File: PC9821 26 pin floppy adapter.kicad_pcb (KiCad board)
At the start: 2 copper layers, 52.7 x 28.6 mm, 3 parts

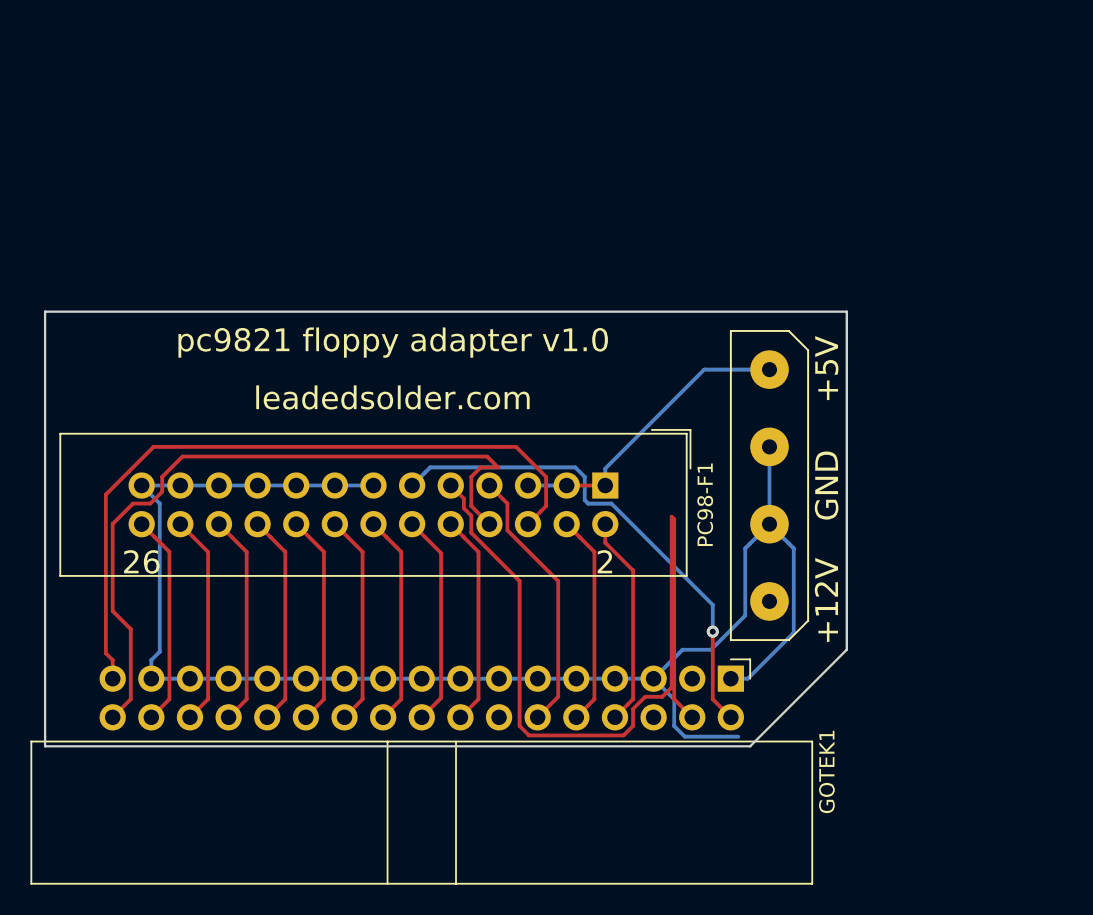
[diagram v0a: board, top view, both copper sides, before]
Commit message: Final version that I just sent off to Osh
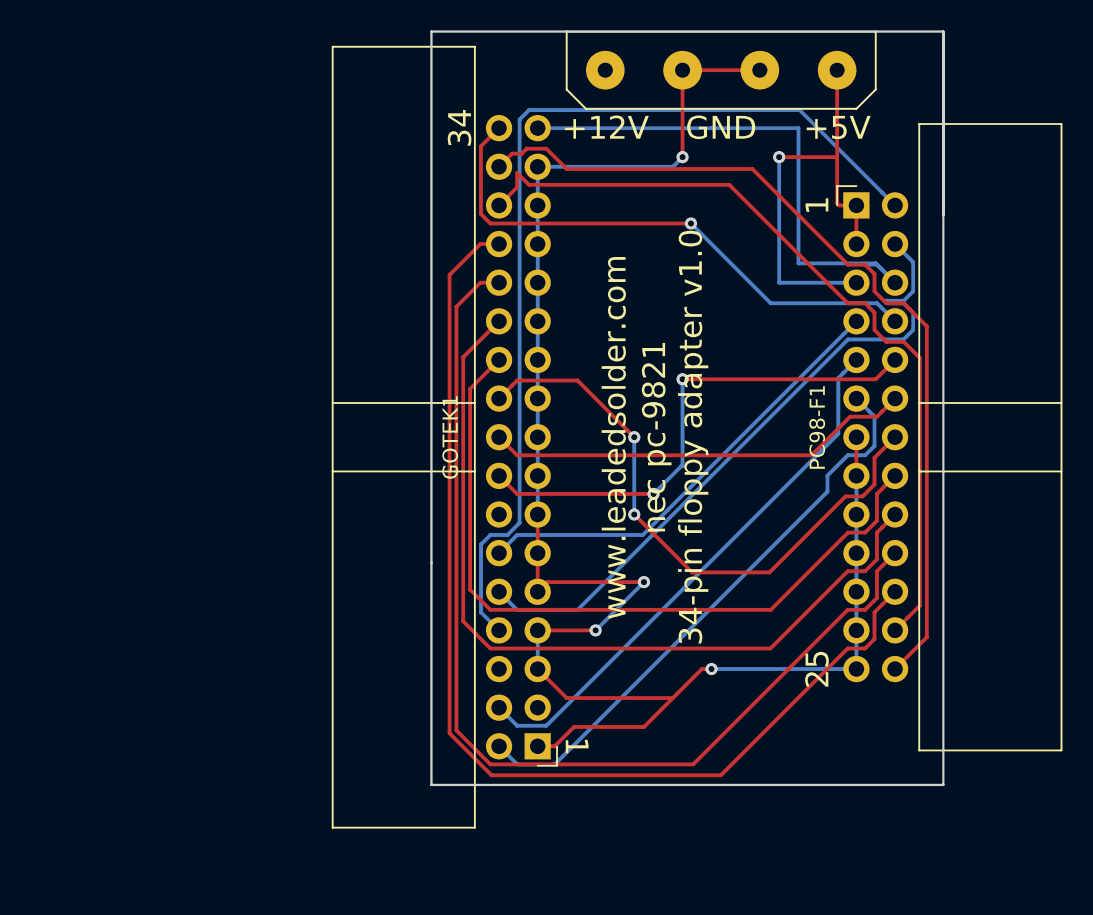
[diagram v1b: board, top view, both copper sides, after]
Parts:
- added G***: LOGO, Logos:skull-silk, B.Cu at (149.9, 92.7)
- PC98-F1: footprint Connector_IDC:IDC-Header_2x13_P2.54mm_Vertical -> Connector_IDC:IDC-Header_2x13_P2.54mm_Horizontal
- moved POWER1 27.5 mm to (151.8, 69.8), turned to 0 degrees
- moved PC98-F1 24.7 mm to (160.7, 78.7), turned to 0 degrees
- moved GOTEK1 13.5 mm to (139.7, 114.3), turned to 180 degrees
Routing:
- net /WRITE_PROTECT: track 13.9 -> 70.7 mm
- net /TRACK_00: track 13.9 -> 67.9 mm
- net /INDEX_OUT: track 13.9 -> 63.3 mm
- net /SIDE: track 13.9 -> 57.5 mm
- net /WRITE_ENABLE: track 13.9 -> 54.5 mm
- net /READ_DATA: track 13.9 -> 53.4 mm
- net /WRITE_DATA: track 13.9 -> 49.1 mm
- net /DRV_SELECT_0: track 13.9 -> 44.5 mm
- net /STEP_PULSE: track 13.9 -> 39.4 mm, vias 0 -> 2
- net /MOTOR_ON: track 13.9 -> 33.5 mm, vias 0 -> 2
- net /HEAD_LOAD: track 54.9 -> 36.1 mm
- net /DIRECTION: track 14.0 -> 28.1 mm
- net /DRV_SELECT_1: track 17.7 -> 29.8 mm
- net /360_300_DRV_0: track 102.5 -> 114.6 mm, vias 0 -> 4
- net /READY_OUT: track 47.4 -> 36.3 mm, vias 0 -> 1
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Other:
- board size 52.7 x 28.6 mm -> 33.7 x 49.5 mm
- board text added: "25"
- board text added: "34"
- board text added: "nec pc-9821 34-pin floppy adapter v1.0"
- board text added: "www.leadedsolder.com"
- board text removed: "2"
- board text removed: "26"
- board text removed: "33"
- board text removed: "key this end"
- board text removed: "leadedsolder.com"
- board text removed: "pc9821 floppy adapter v1.0"
